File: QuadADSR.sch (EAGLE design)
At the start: 67 parts, among them IC1 74AC32D, IC5 MCP6004D, Q1 20MHz, T1 2N3904, T2 2N3904, T3 2N3904, T4 2N3904, U1 ATMEGA328P, U2 DUAL_OPAMP, U3 7805, U4 4051

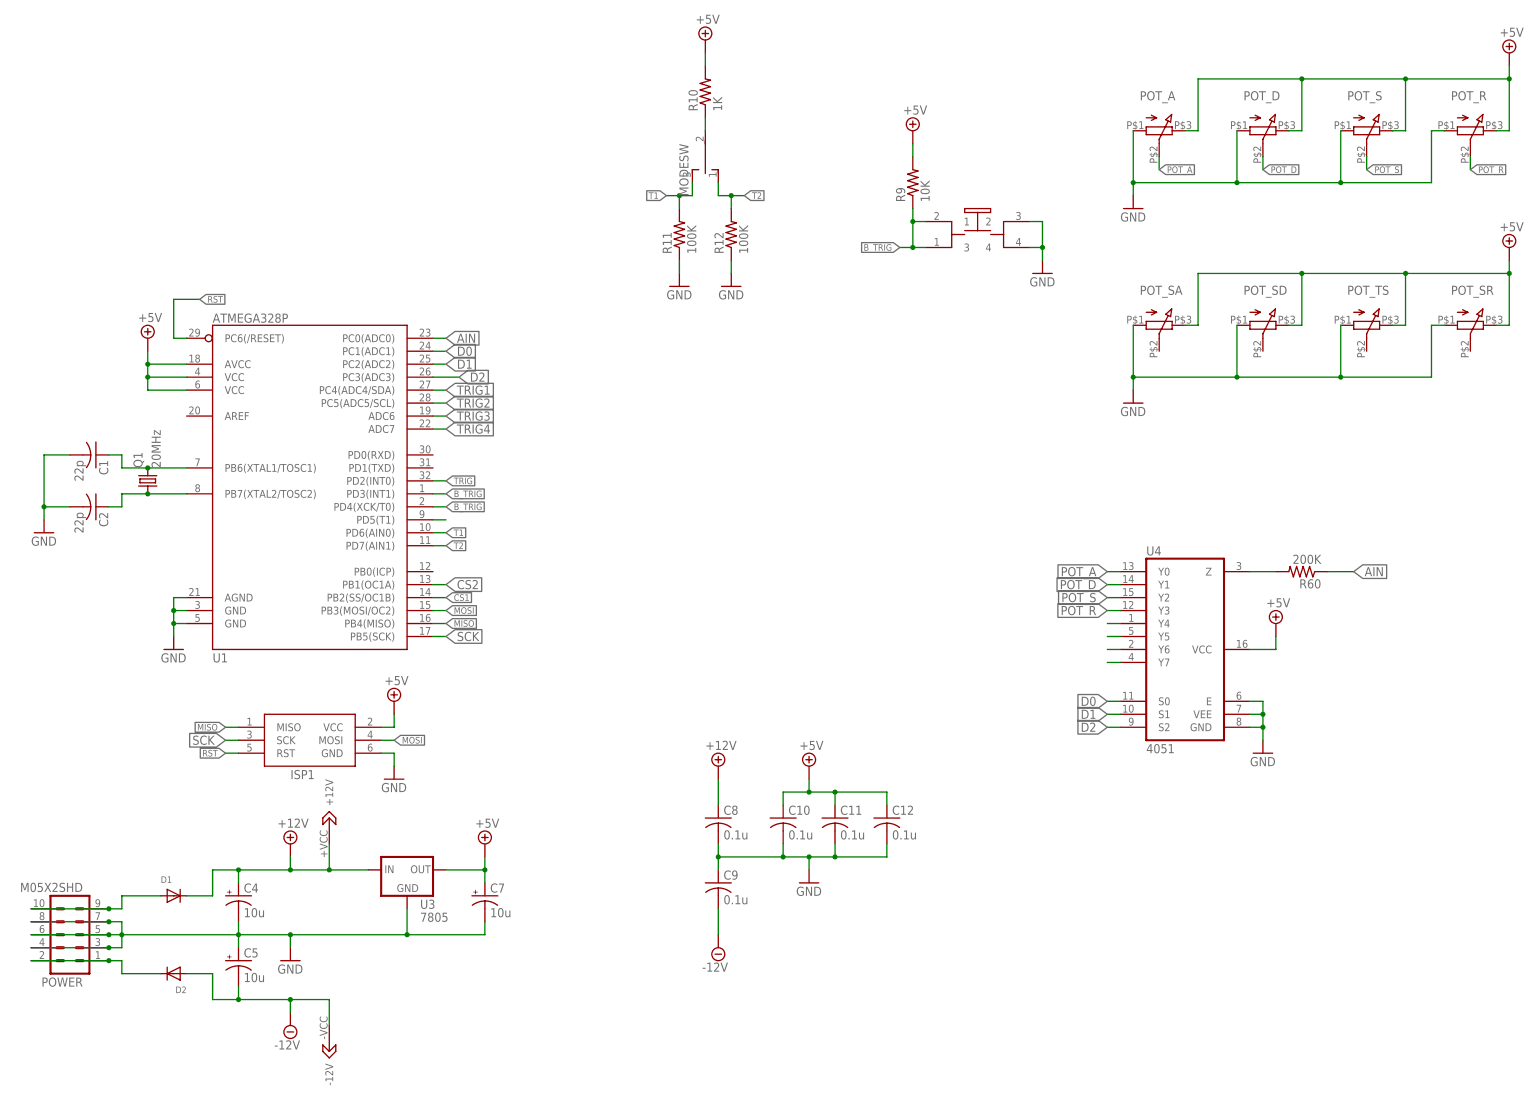
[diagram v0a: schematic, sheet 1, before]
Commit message: Moved a few thigs round
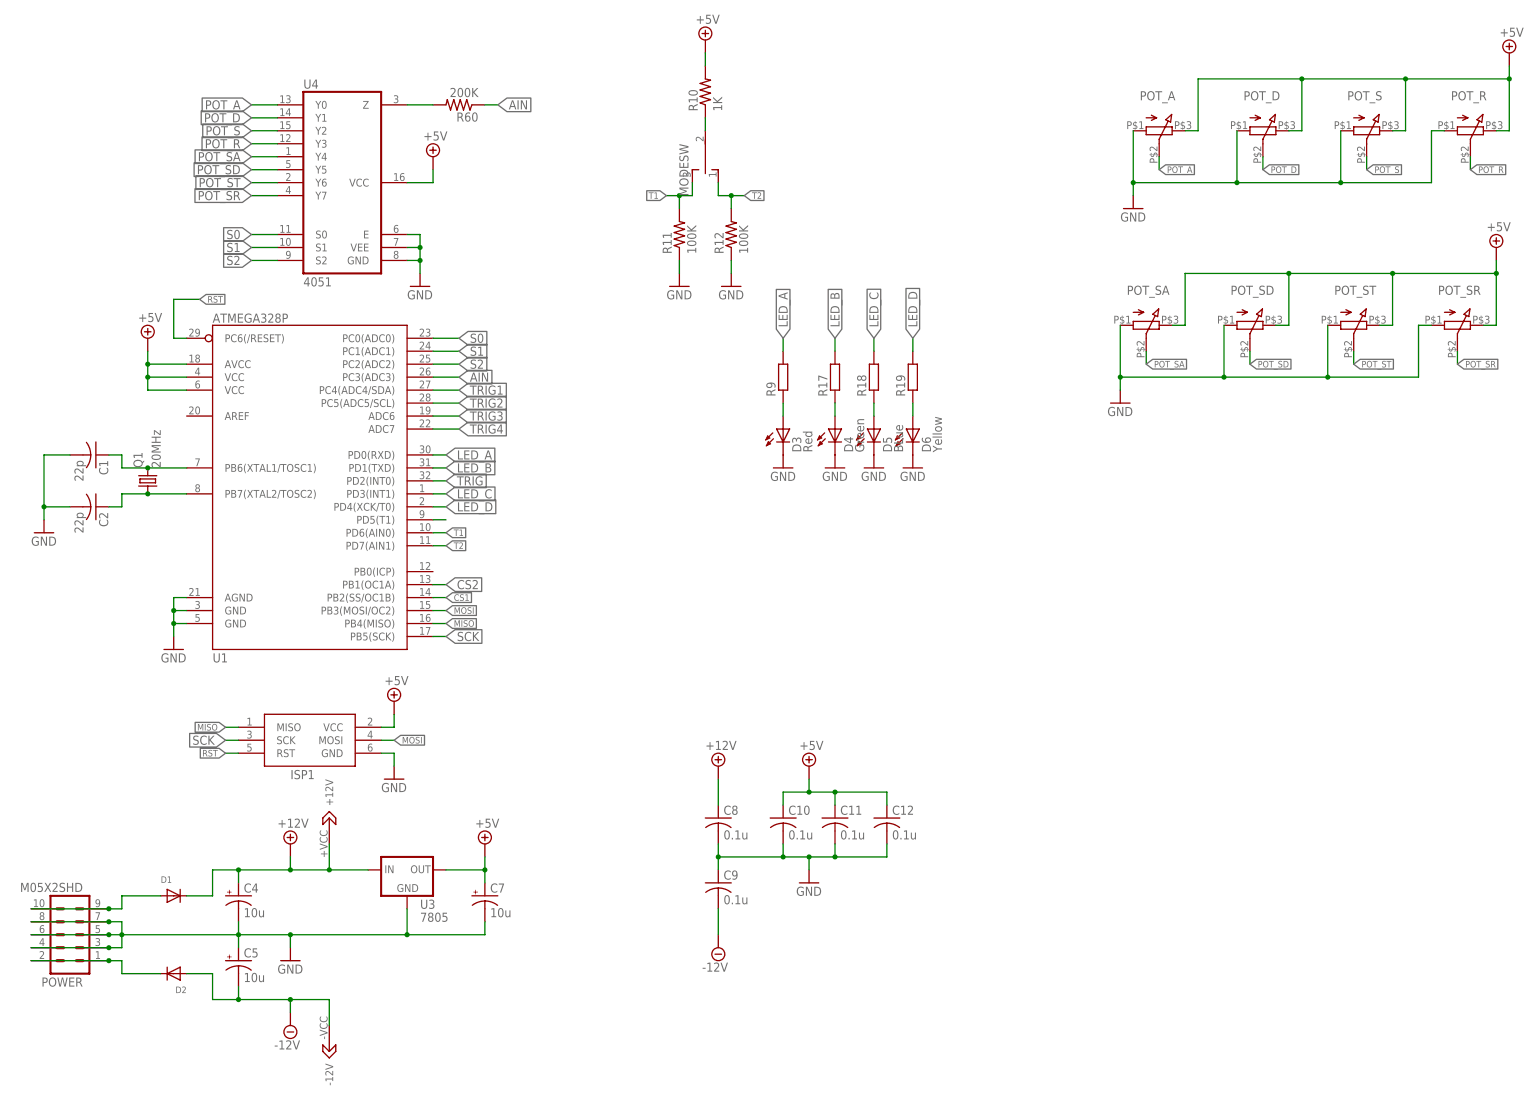
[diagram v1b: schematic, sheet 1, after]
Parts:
- removed BUT: PB6149L-5, INSTRUO:PB6149L-5
- removed POT_TS: Q-POT, INSTRUO:Q-POT
- added D3: Red, led:LED5MM
- added D4: Green, led:LED5MM
- added D5: BLue, led:LED5MM
- added D6: Yellow, led:LED5MM
- added POT_ST: Q-POT, INSTRUO:Q-POT
- added R17, R18, R19: (no value), resistor:R-EU_R0805
- R9: value 10K -> (none); device rcl:R-US_R0805 -> resistor:R-EU_R0805
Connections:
- removed net B_TRIG: BUTG$1.1, BUTG$1.3, R9.1, U1.PD3(INT1), U1.PD4(XCK/T0)
- removed net D0: U1.PC1(ADC1), U4.S0
- removed net D1: U1.PC2(ADC2), U4.S1
- removed net D2: U1.PC3(ADC3), U4.S2
- removed net N$23: U4.Y4
- removed net N$24: U4.Y5
- removed net N$26: U4.Y6
- removed net N$27: U4.Y7
- new net LED_A: R9.2, U1.PD0(RXD)
- new net LED_B: R17.2, U1.PD1(TXD)
- new net LED_C: R18.2, U1.PD3(INT1)
- new net LED_D: R19.2, U1.PD4(XCK/T0)
- new net N$19: D3.A, R9.1
- new net N$20: D4.A, R17.1
- new net N$21: D5.A, R18.1
- new net N$22: D6.A, R19.1
- new net POT_SA: POT_SA.2, U4.Y4
- new net POT_SD: POT_SD.2, U4.Y5
- new net POT_SR: POT_SR.2, U4.Y7
- new net POT_ST: POT_ST.2, U4.Y6
- new net S0: U1.PC0(ADC0), U4.S0
- new net S1: U1.PC1(ADC1), U4.S1
- new net S2: U1.PC2(ADC2), U4.S2
- net +5V: now also POT_ST.3; no longer POT_TS.3, R9.2
- net AIN: now also U1.PC3(ADC3); no longer U1.PC0(ADC0)
- net GND: now also D3.C, D4.C, D5.C, D6.C, POT_ST.1; no longer BUTG$1.2, BUTG$1.4, POT_TS.1
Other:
- moved on the sheet: POT_SA, POT_SD, POT_SR, R60, U4
